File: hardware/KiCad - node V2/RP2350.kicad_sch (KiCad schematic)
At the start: 92 parts, among them J1 Input, J2 Output, J3 USB_C_Receptacle_USB2.0_14P, J4 Screw_Terminal_01x08, SW1 BOOTSEL, U1 RP2350A, U2 THVD1450D, U3 ADXL355BEZ, U4 TPS2121RUXR, U5 USBLC6-2SC6, U6 TLV75733PDBV, U7 W25Q128JVS, U8 TPS7A20xxxDBV

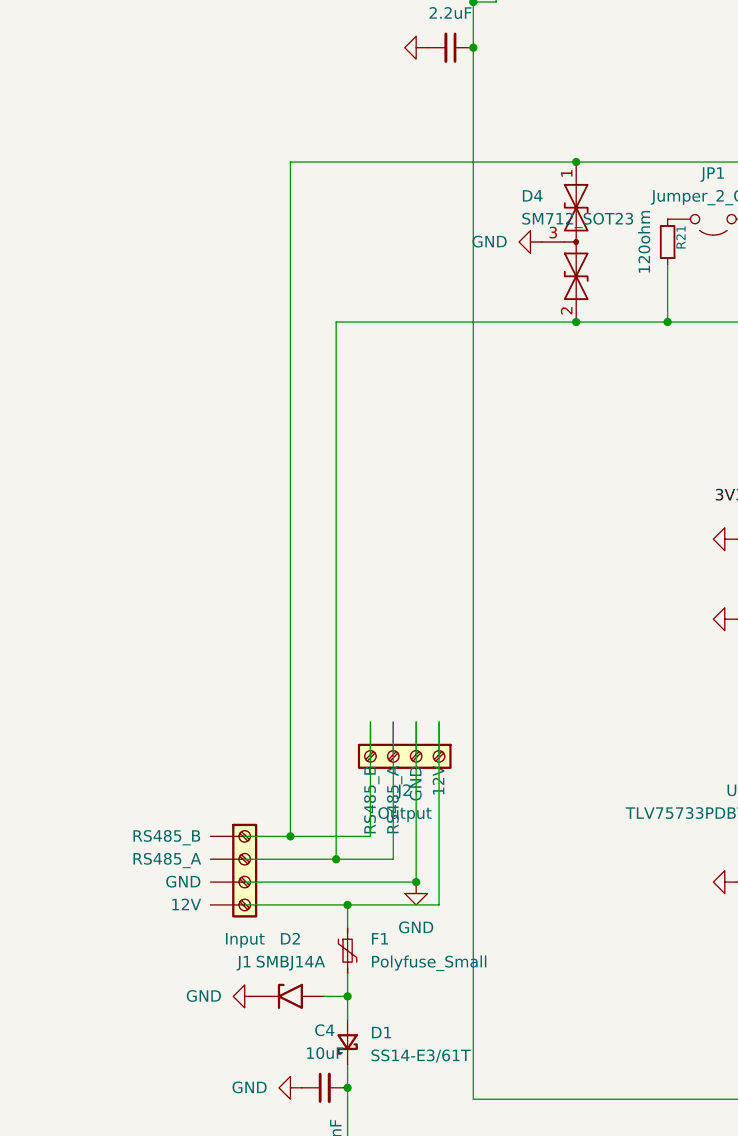
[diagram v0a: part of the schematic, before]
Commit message: KiCad: J1 terminal update
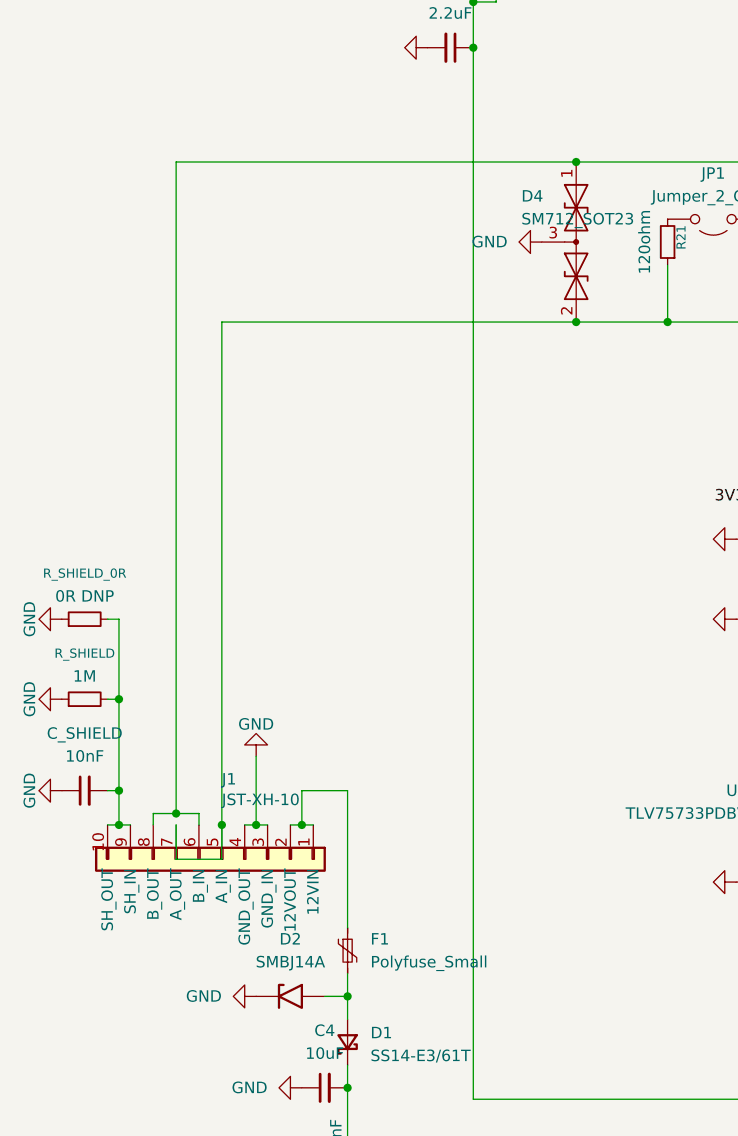
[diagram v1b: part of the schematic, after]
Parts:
- removed J1: Input, TerminalBlock_RND:TerminalBlock_RND_205-00278_1x04_P5.00mm_Vertical, symbol Connector:Screw_Terminal_01x04
- removed J2: Output, symbol Connector:Screw_Terminal_01x04
- added C_SHIELD: 10nF, Capacitor_SMD:C_0805_2012Metric, symbol Device:C_Small
- added J1: JST-XH-10, footprints:CONN-TH_10P-P2.50_B10B-XH-A-LF-SN, symbol Connector_Generic:Conn_01x10
- added R_SHIELD: 1M, Resistor_SMD:R_0603_1608Metric, symbol Device:R_Small
- added R_SHIELD_0R: 0R DNP, Resistor_SMD:R_0805_2012Metric, symbol Device:R_Small
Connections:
- net GND: now also C_SHIELD.1, J1.3 (GND_IN), J1.4 (GND_OUT), R_SHIELD.1, R_SHIELD_0R.1
- net at D4.2 (A2), R21.1, U2.6 (A): now also J1.5 (A_IN), J1.7 (A_OUT)
- net at D4.1 (A1), JP1.1 (A), U2.7 (B): now also J1.6 (B_IN), J1.8 (B_OUT)
- net at F1.1: now also J1.1 (12VIN), J1.2 (12VOUT)
- new net: C_SHIELD.2, J1.10 (SH_OUT), J1.9 (SH_IN), R_SHIELD.2, R_SHIELD_0R.2
